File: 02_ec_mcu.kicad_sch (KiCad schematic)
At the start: 48 parts, among them J16 Case power/reset button harne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, J4 TC2030 Cortex SWD: VTref/SWDI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, SW1 Reset, SW4 BOOT0 (DFU), U4 STM32F407VGTx, U44 TCA9539PWR resettable source 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, U46 SN74LVC1G08DBVR EC-reset-qual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, U5 TPS54202DDC, Y1 J32SMX-K-F-G-I-8M0 8MHz CL8pF, Y2 X1A000141000612 32.768kHz CL6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

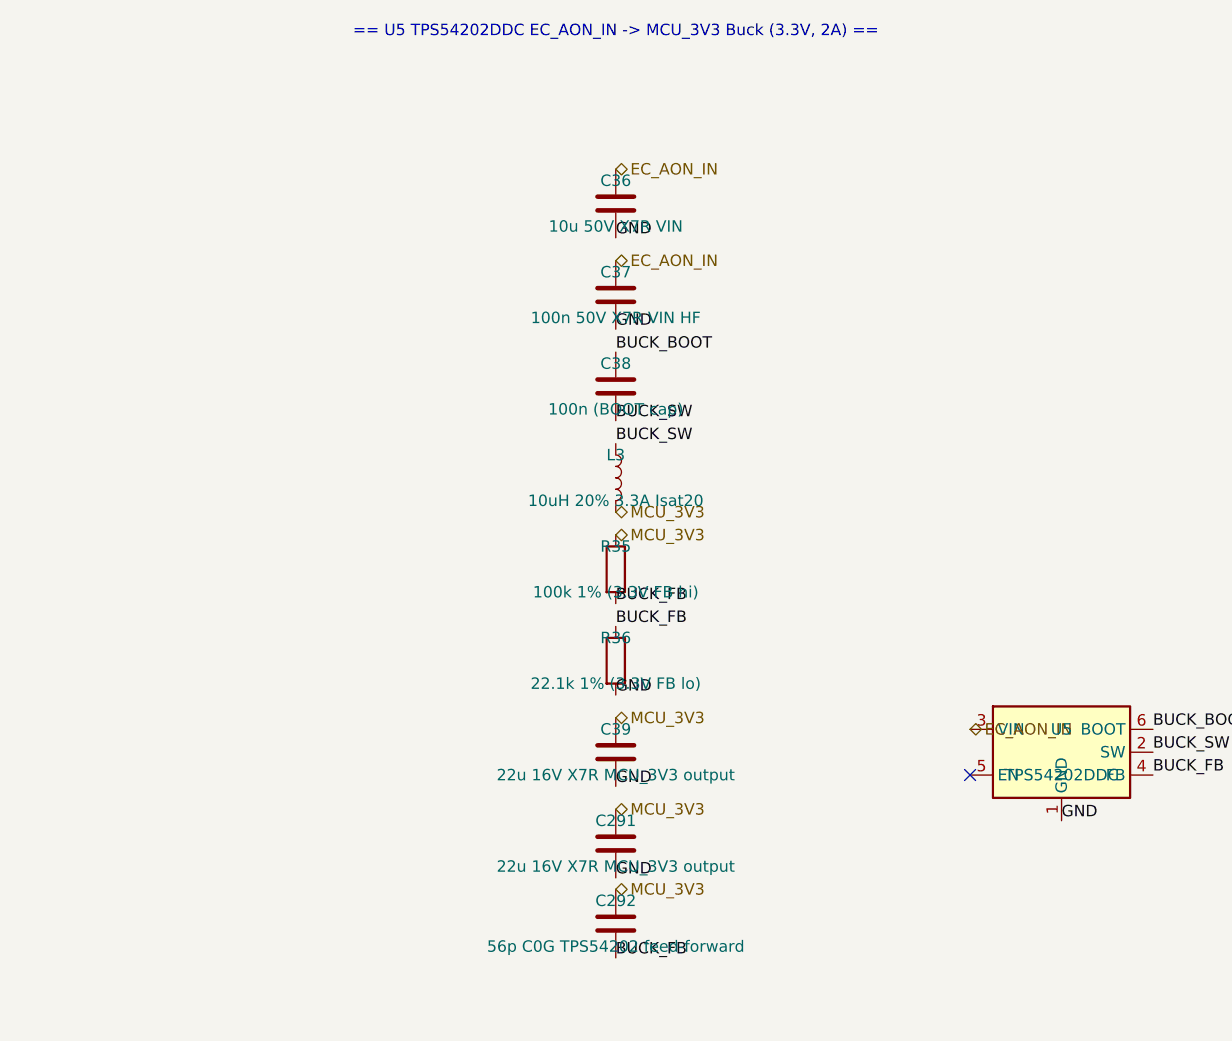
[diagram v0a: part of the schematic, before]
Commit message: fix the center layout and more board issues
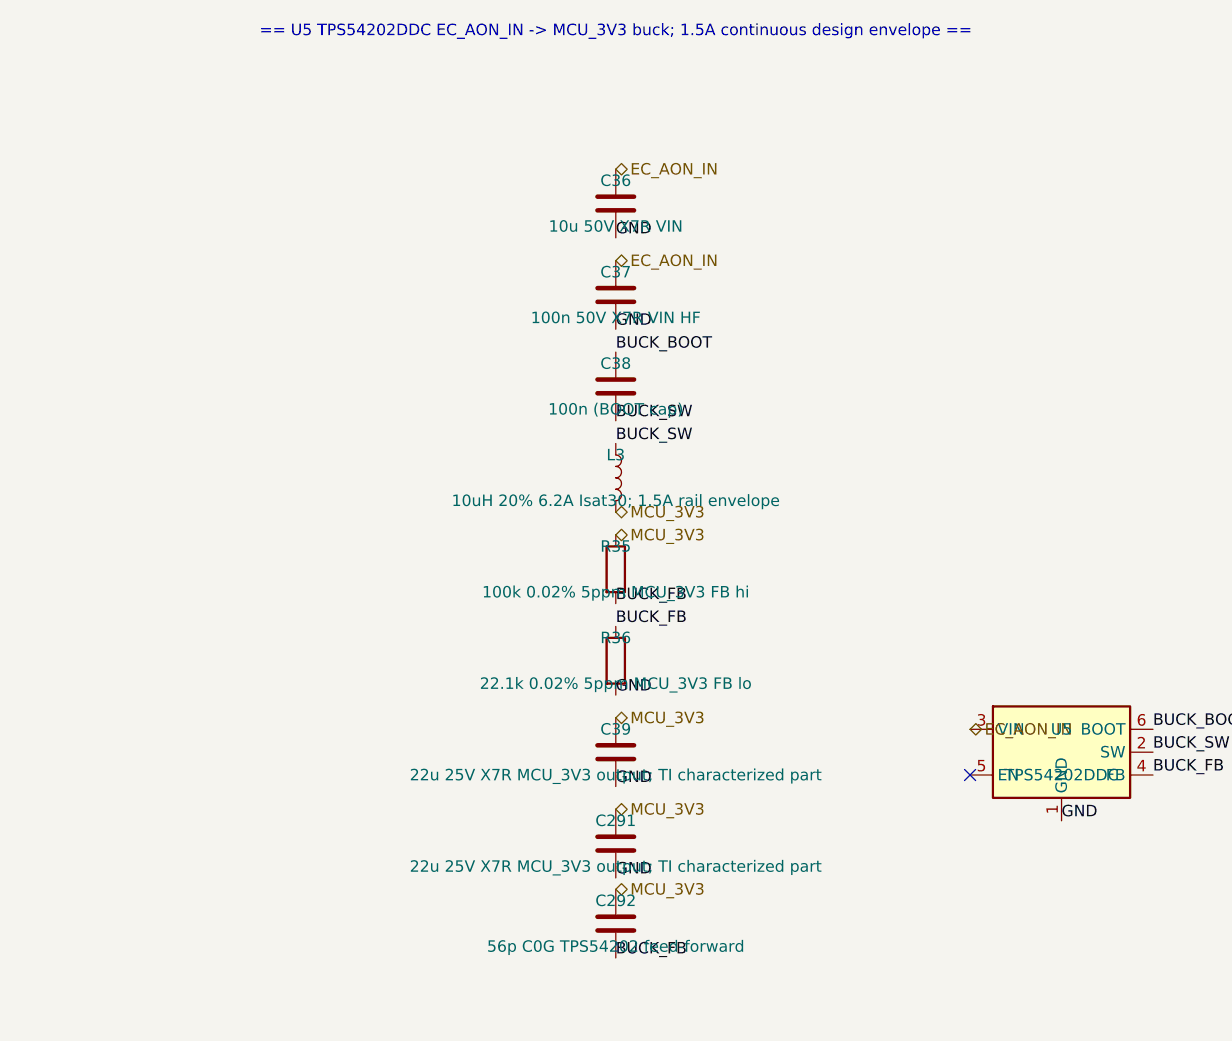
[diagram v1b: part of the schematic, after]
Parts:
- C291, C39: value 22u 16V X7R MCU_3V3 output -> 22u 25V X7R MCU_3V3 output; TI characterized part; footprint Capacitor_SMD:C_1206_3216Metric -> Capacitor_SMD:C_1210_3225Metric; MPN GRM31CZ71C226ME15L -> GRM32ER71E226KE15L
- L3: value 10uH 20% 3.3A Isat20 -> 10uH 20% 6.2A Isat30; 1.5A rail envelope; footprint ducktop2:Coilcraft_XGL5030 -> ducktop2:Coilcraft_XGL6030; MPN XGL5030-103MEC -> XGL6030-103MEC
- R35: value 100k 1% (3.3V FB hi) -> 100k 0.02% 5ppm MCU_3V3 FB hi; MPN RC0603FR-07100KL -> TNPU0603100KHZEN00; Manufacturer Yageo -> Vishay
- R36: value 22.1k 1% (3.3V FB lo) -> 22.1k 0.02% 5ppm MCU_3V3 FB lo; MPN RC0603FR-0722K1L -> TNPU060322K1HZEN00; Manufacturer Yageo -> Vishay
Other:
- note added: "== U5 TPS54202DDC EC_AON_IN -> MCU_3V3 buck; 1.5A continuous design envelope =="
- note removed: "== U5 TPS54202DDC EC_AON_IN -> MCU_3V3 Buck (3.3V, 2A) =="
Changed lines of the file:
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@@
   (effects (font (size 1.27 1.27)) (justify left bottom))
 )
-(text "== U5 TPS54202DDC EC_AON_IN -> MCU_3V3 Buck (3.3V, 2A) ==" (at 650.24 20.32 0) (effects (font (size 1.27 1.27))))
+(text "== U5 TPS54202DDC EC_AON_IN -> MCU_3V3 buck; 1.5A continuous design envelope ==" (at 650.24 20.32 0) (effects (font (size 1.27 1.27))))
 (symbol
   (lib_id "ducktop2:TPS54202DDC")
@@
   (dnp no)
   (property "Reference" "L3" (at 650.24 67.31 0) (effects (font (size 1.27 1.27))))
-  (property "Value" "10uH 20% 3.3A Isat20" (at 650.24 72.39 0) (effects (font (size 1.27 1.27))))
-  (property "Footprint" "ducktop2:Coilcraft_XGL5030" (at 650.24 69.85 0) (effects (font (size 1.27 1.27)) (hide yes)))
+  (property "Value" "10uH 20% 6.2A Isat30; 1.5A rail envelope" (at 650.24 72.39 0) (effects (font (size 1.27 1.27))))
+  (property "Footprint" "ducktop2:Coilcraft_XGL6030" (at 650.24 69.85 0) (effects (font (size 1.27 1.27)) (hide yes)))
   (property "Datasheet" "" (at 650.24 69.85 0) (effects (font (size 1.27 1.27)) (hide yes)))
   (property "Manufacturer" "Coilcraft" (at 650.24 69.85 0) (effects (font (size 1.27 1.27)) (hide yes)))
-  (property "MPN" "XGL5030-103MEC" (at 650.24 69.85 0) (effects (font (size 1.27 1.27)) (hide yes)))
-  (property "Datasheet" "https://www.coilcraft.com/getmedia/e64ac115-95f2-45c7-b798-1b3769b91583/xgl5030.pdf" (at 650.24 69.85 0) (effects (font (size 1.27 1.27)) (hide yes)))
+  (property "MPN" "XGL6030-103MEC" (at 650.24 69.85 0) (effects (font (size 1.27 1.27)) (hide yes)))
+  (property "Datasheet" "https://www.coilcraft.com/getmedia/9bfb2606-51aa-49a6-98ad-d20f3504c8ae/xgl6030.pdf" (at 650.24 69.85 0) (effects (font (size 1.27 1.27)) (hide yes)))
   (pin "1")
   (pin "2")
@@
   (dnp no)
   (property "Reference" "R35" (at 650.24 77.47 0) (effects (font (size 1.27 1.27))))
-  (property "Value" "100k 1% (3.3V FB hi)" (at 650.24 82.55 0) (effects (font (size 1.27 1.27))))
+  (property "Value" "100k 0.02% 5ppm MCU_3V3 FB hi" (at 650.24 82.55 0) (effects (font (size 1.27 1.27))))
   (property "Footprint" "Resistor_SMD:R_0603_1608Metric" (at 650.24 80.01 0) (effects (font (size 1.27 1.27)) (hide yes)))
   (property "Datasheet" "" (at 650.24 80.01 0) (effects (font (size 1.27 1.27)) (hide yes)))
-  (property "Manufacturer" "Yageo" (at 650.24 80.01 0) (effects (font (size 1.27 1.27)) (hide yes)))
-  (property "MPN" "RC0603FR-07100KL" (at 650.24 80.01 0) (effects (font (size 1.27 1.27)) (hide yes)))
+  (property "Manufacturer" "Vishay" (at 650.24 80.01 0) (effects (font (size 1.27 1.27)) (hide yes)))
+  (property "MPN" "TNPU0603100KHZEN00" (at 650.24 80.01 0) (effects (font (size 1.27 1.27)) (hide yes)))
   (pin "1")
   (pin "2")
@@
   (dnp no)
   (property "Reference" "R36" (at 650.24 87.63 0) (effects (font (size 1.27 1.27))))
-  (property "Value" "22.1k 1% (3.3V FB lo)" (at 650.24 92.71 0) (effects (font (size 1.27 1.27))))
+  (property "Value" "22.1k 0.02% 5ppm MCU_3V3 FB lo" (at 650.24 92.71 0) (effects (font (size 1.27 1.27))))
   (property "Footprint" "Resistor_SMD:R_0603_1608Metric" (at 650.24 90.17 0) (effects (font (size 1.27 1.27)) (hide yes)))
   (property "Datasheet" "" (at 650.24 90.17 0) (effects (font (size 1.27 1.27)) (hide yes)))
-  (property "Manufacturer" "Yageo" (at 650.24 90.17 0) (effects (font (size 1.27 1.27)) (hide yes)))
-  (property "MPN" "RC0603FR-0722K1L" (at 650.24 90.17 0) (effects (font (size 1.27 1.27)) (hide yes)))
+  (property "Manufacturer" "Vishay" (at 650.24 90.17 0) (effects (font (size 1.27 1.27)) (hide yes)))
+  (property "MPN" "TNPU060322K1HZEN00" (at 650.24 90.17 0) (effects (font (size 1.27 1.27)) (hide yes)))
   (pin "1")
   (pin "2")
@@
   (dnp no)
   (property "Reference" "C39" (at 650.24 97.79 0) (effects (font (size 1.27 1.27))))
-  (property "Value" "22u 16V X7R MCU_3V3 output" (at 650.24 102.87 0) (effects (font (size 1.27 1.27))))
-  (property "Footprint" "Capacitor_SMD:C_1206_3216Metric" (at 650.24 100.33 0) (effects (font (size 1.27 1.27)) (hide yes)))
+  (property "Value" "22u 25V X7R MCU_3V3 output; TI characterized part" (at 650.24 102.87 0) (effects (font (size 1.27 1.27))))
+  (property "Footprint" "Capacitor_SMD:C_1210_3225Metric" (at 650.24 100.33 0) (effects (font (size 1.27 1.27)) (hide yes)))
   (property "Datasheet" "" (at 650.24 100.33 0) (effects (font (size 1.27 1.27)) (hide yes)))
   (property "Manufacturer" "Murata" (at 650.24 100.33 0) (effects (font (size 1.27 1.27)) (hide yes)))
-  (property "MPN" "GRM31CZ71C226ME15L" (at 650.24 100.33 0) (effects (font (size 1.27 1.27)) (hide yes)))
+  (property "MPN" "GRM32ER71E226KE15L" (at 650.24 100.33 0) (effects (font (size 1.27 1.27)) (hide yes)))
   (pin "1")
   (pin "2")
@@
   (dnp no)
   (property "Reference" "C291" (at 650.24 107.95 0) (effects (font (size 1.27 1.27))))
-  (property "Value" "22u 16V X7R MCU_3V3 output" (at 650.24 113.03 0) (effects (font (size 1.27 1.27))))
-  (property "Footprint" "Capacitor_SMD:C_1206_3216Metric" (at 650.24 110.49 0) (effects (font (size 1.27 1.27)) (hide yes)))
+  (property "Value" "22u 25V X7R MCU_3V3 output; TI characterized part" (at 650.24 113.03 0) (effects (font (size 1.27 1.27))))
+  (property "Footprint" "Capacitor_SMD:C_1210_3225Metric" (at 650.24 110.49 0) (effects (font (size 1.27 1.27)) (hide yes)))
   (property "Datasheet" "" (at 650.24 110.49 0) (effects (font (size 1.27 1.27)) (hide yes)))
   (property "Manufacturer" "Murata" (at 650.24 110.49 0) (effects (font (size 1.27 1.27)) (hide yes)))
-  (property "MPN" "GRM31CZ71C226ME15L" (at 650.24 110.49 0) (effects (font (size 1.27 1.27)) (hide yes)))
-  (pin "1")
-  (pin "2")
+  (property "MPN" "GRM32ER71E226KE15L" (at 650.24 110.49 0) (effects (font (size 1.27 1.27)) (hide yes)))
+  (pin "1")
+  (pin "2")
